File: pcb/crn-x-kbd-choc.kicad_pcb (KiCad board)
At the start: 2 copper layers, 149.2 x 93.1 mm, 58 parts, among them SW1 SW_PUSH, SW10 SW_PUSH, SW11 SW_PUSH, SW12 SW_PUSH, SW13 SW_PUSH, SW14 SW_PUSH, SW15 SW_PUSH, SW16 SW_PUSH, SW17 SW_PUSH, SW18 SW_PUSH, SW19 SW_PUSH, SW2 SW_PUSH, SW20 SW_PUSH, SW21 SW_PUSH, SW3 SW_PUSH, SW4 SW_PUSH, SW5 SW_PUSH, SW6 SW_PUSH, SW7 SW_PUSH, SW8 SW_PUSH, SW9 SW_PUSH, U1 xiao-ble, U4 xiao-ble

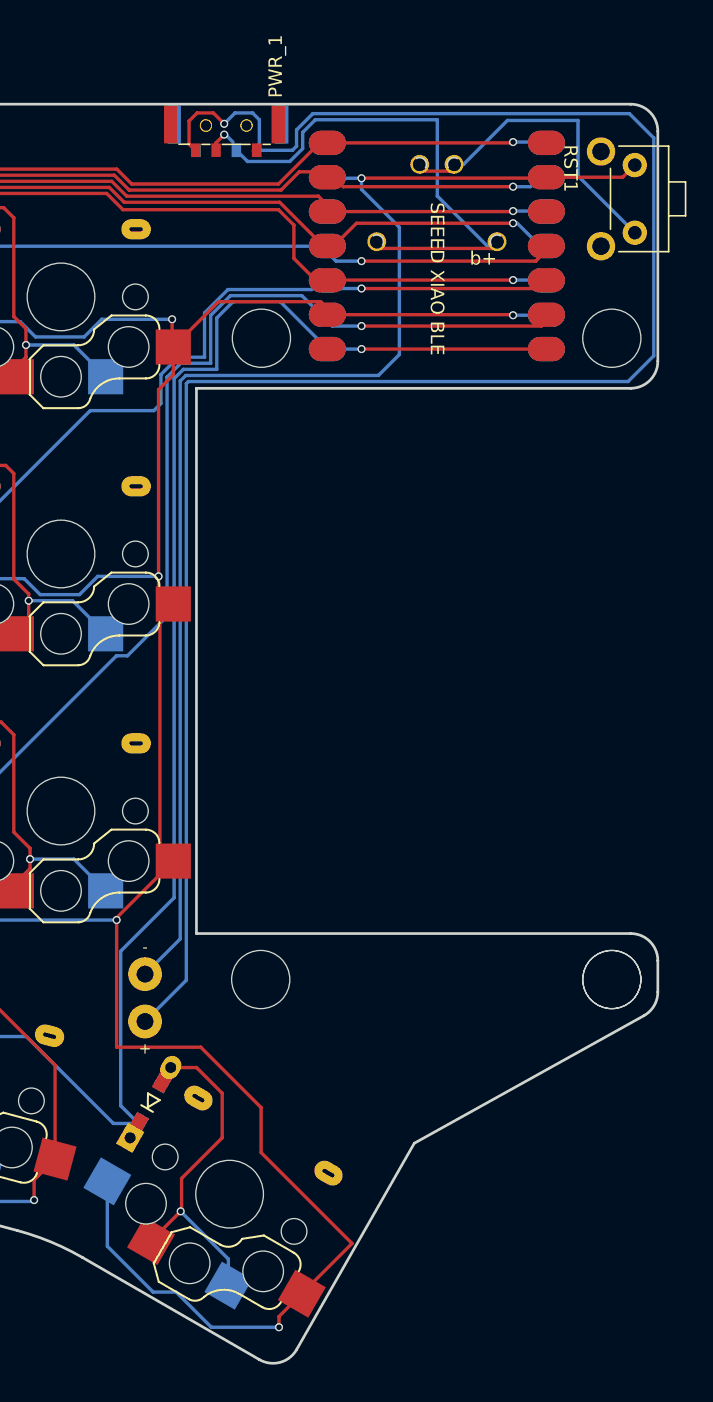
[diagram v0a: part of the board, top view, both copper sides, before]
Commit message: other
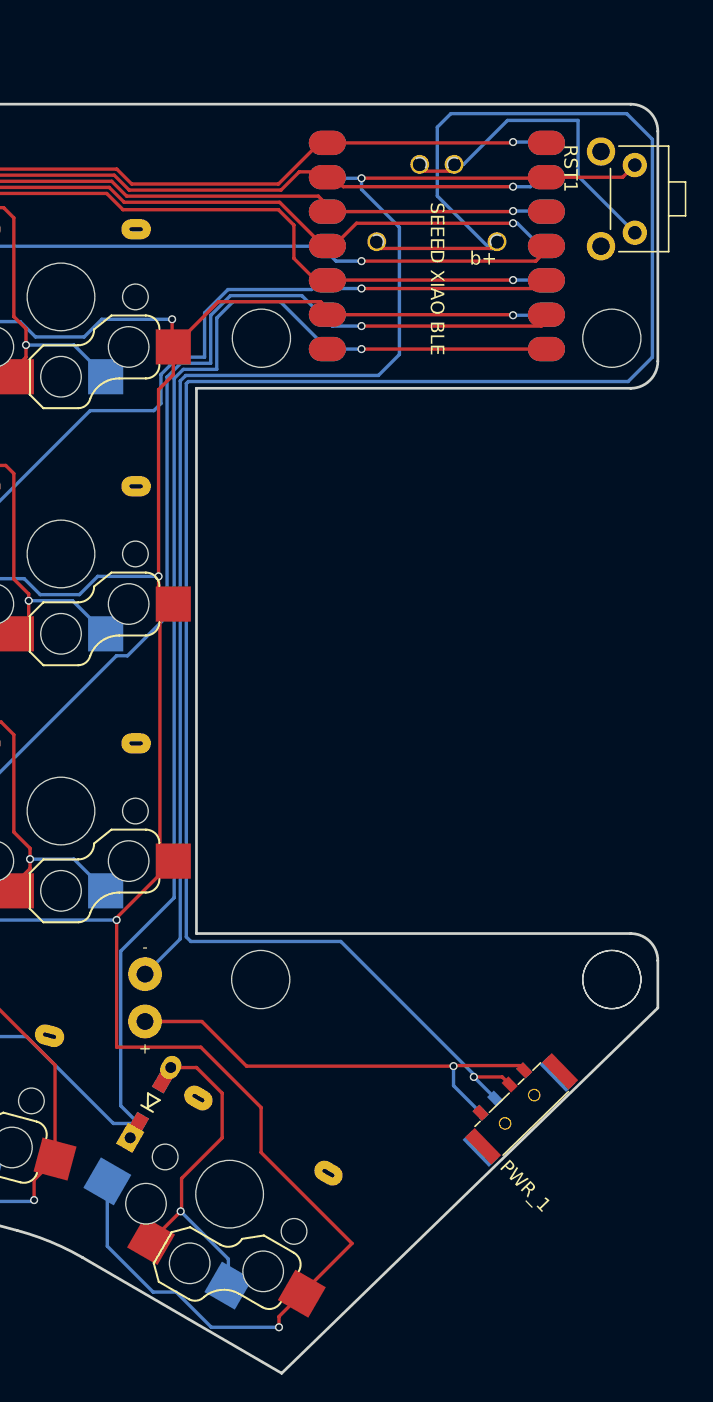
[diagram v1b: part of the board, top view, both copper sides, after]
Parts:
- moved PWR_1 79.4 mm to (149.4, 107.2), turned to 134.2 degrees
- moved PWR_2 78.1 mm to (154.7, 102.0), turned to 134.2 degrees
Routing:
- net BAT+: track 42.8 -> 163.3 mm
- net VBAT: track 143.5 -> 33.8 mm
- net unconnected-(PWR_2-A-Pad1): track 0.00 -> 0.50 mm
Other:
- board size 149.2 x 93.1 mm -> 149.2 x 93.8 mm
